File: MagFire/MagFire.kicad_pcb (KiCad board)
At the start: 2 copper layers, 1 part

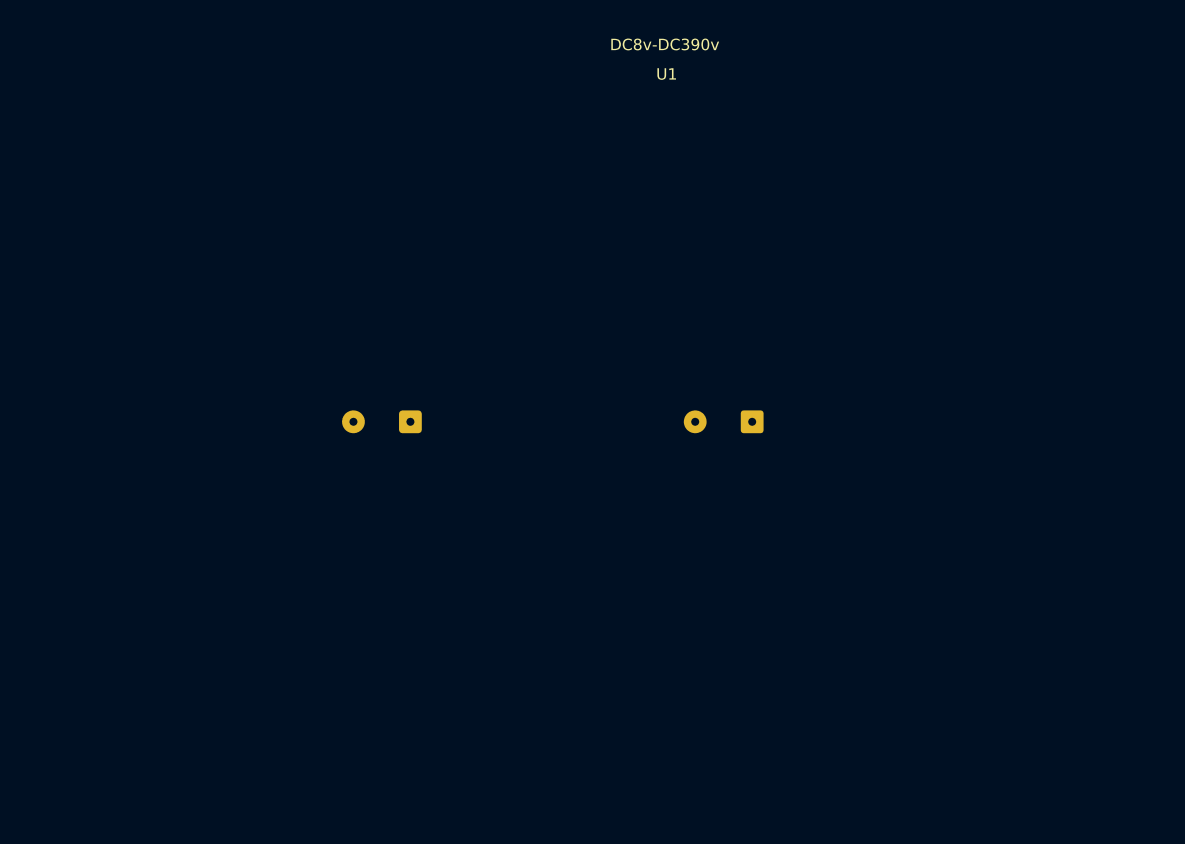
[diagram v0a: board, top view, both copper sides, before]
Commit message: update model and pcb and journal
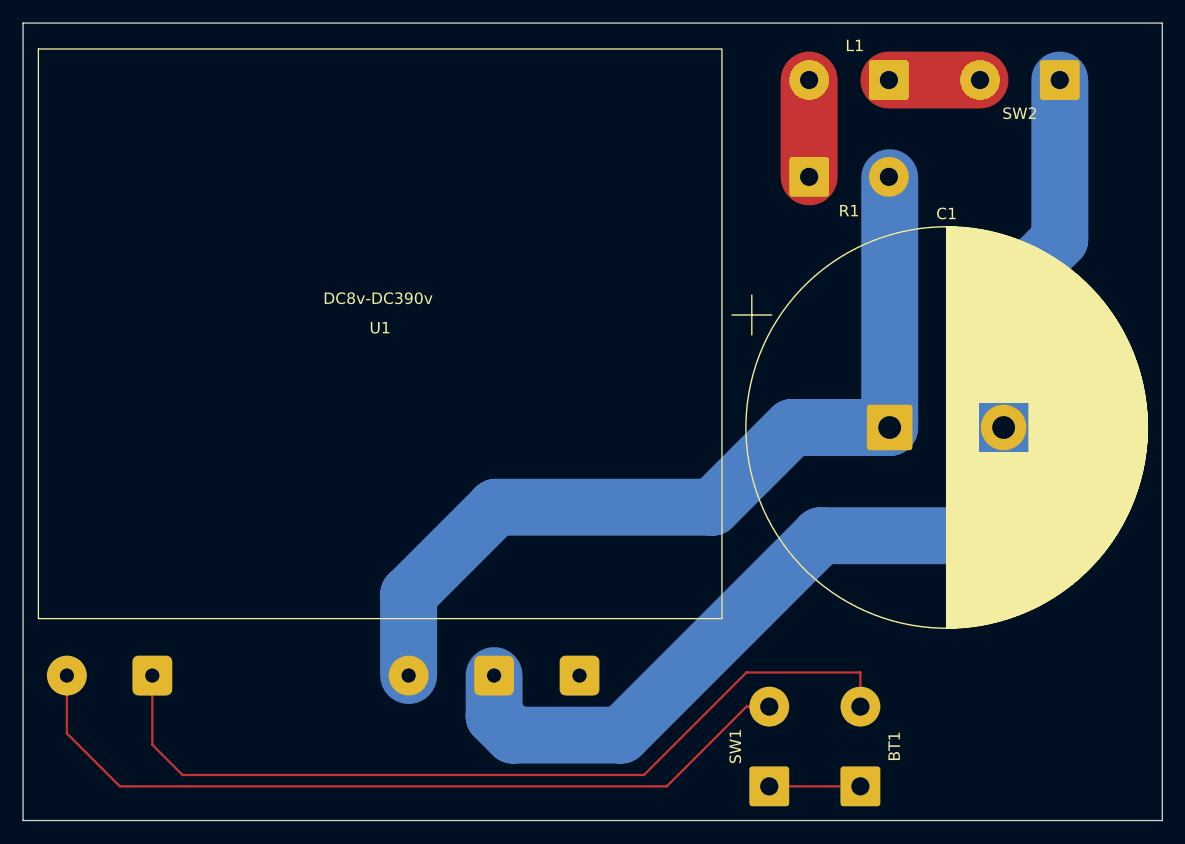
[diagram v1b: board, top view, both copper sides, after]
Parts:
- added BT1: Battery, Connector_Wire:SolderWire-0.75sqmm_1x02_P7mm_D1.25mm_OD3.5mm, F.Cu at (146.5, 142.5)
- added C1: C_US, Capacitor_THT:CP_Radial_D35.0mm_P10.00mm_SnapIn, F.Cu at (149.1, 111.0)
- added L1: L, Connector_Wire:SolderWire-0.75sqmm_1x02_P7mm_D1.25mm_OD3.5mm, F.Cu at (149.0, 80.5)
- added R1: R_US, Connector_Wire:SolderWire-0.75sqmm_1x02_P7mm_D1.25mm_OD3.5mm, F.Cu at (142.0, 89.0)
- added SW1: SW_Push, Connector_Wire:SolderWire-0.75sqmm_1x02_P7mm_D1.25mm_OD3.5mm, F.Cu at (138.5, 142.5)
- added SW2: SW_Push, Connector_Wire:SolderWire-0.75sqmm_1x02_P7mm_D1.25mm_OD3.5mm, F.Cu at (164.0, 80.5)
- U1: footprint KS_Maker:DC-DC390v_transformer_2 -> KS_Maker:DC-DC390v_transformer_3
- moved U1 33.6 mm to (104.3, 102.8)
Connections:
- U1 pad 1: unconnected-(U1-IN+-Pad1) -> Net-(U1-IN+)
- U1 pad 2: unconnected-(U1-IN--Pad2) -> Net-(BT1--)
- U1 pad 3: unconnected-(U1-OUT+-Pad3) -> Net-(U1-OUT+)
- U1 pad 4: unconnected-(U1-OUT-Pad4) -> Net-(U1-OUT)
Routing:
- net Net-(U1-OUT): track 0.00 -> 96.5 mm
- net Net-(U1-OUT+): track 0.00 -> 77.5 mm
- net Net-(BT1--): track 0.00 -> 76.5 mm
- net Net-(U1-IN+): track 0.00 -> 71.6 mm
- net Net-(L1-Pad2): track 0.00 -> 8.50 mm
- net Net-(L1-Pad1): track 0.00 -> 8.00 mm
- net Net-(BT1-+): track 0.00 -> 8.00 mm
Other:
- board outline added: 100 x 70 mm

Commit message: update everything
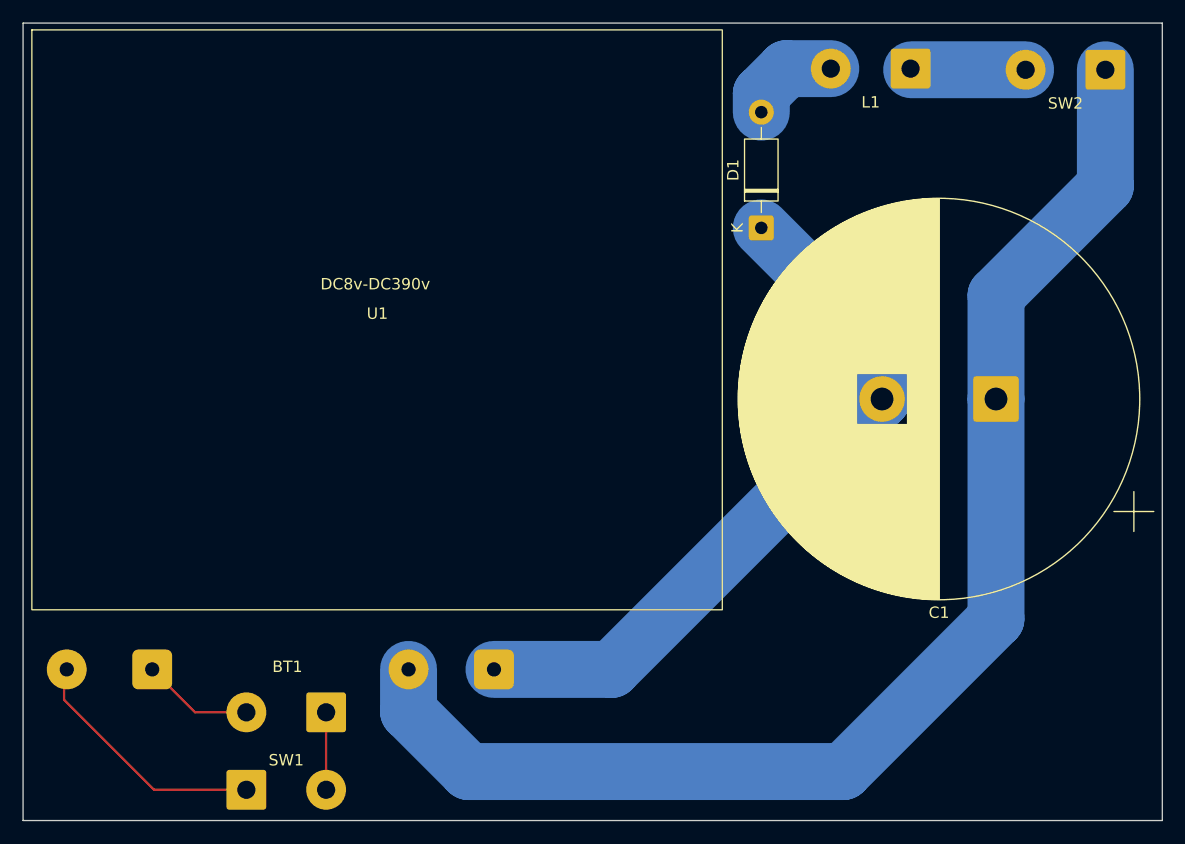
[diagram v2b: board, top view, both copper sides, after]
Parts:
- removed R1: R_US, Connector_Wire:SolderWire-0.75sqmm_1x02_P7mm_D1.25mm_OD3.5mm
- added D1: 1N4007, Diode_THT:D_DO-41_SOD81_P10.16mm_Horizontal, F.Cu at (137.8, 93.5)
- U1: footprint KS_Maker:DC-DC390v_transformer_3 -> KS_Maker:DC-DC390v_transformer_2
- moved BT1 47.3 mm to (99.6, 136.0), turned to 180 degrees
- moved SW1 45.9 mm to (92.6, 142.8), turned to 0 degrees
- moved C1 9.66 mm to (158.4, 108.5), turned to 180 degrees
- moved SW2 4.10 mm to (168.0, 79.6)
- moved L1 2.15 mm to (150.9, 79.5)
- moved U1 1.30 mm to (104.1, 101.5)
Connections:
- C1 pad 2: Net-(U1-OUT) -> Net-(D1-K)
- SW1 pad 1: Net-(BT1-+) -> Net-(U1-IN+)
- SW1 pad 2: Net-(U1-IN+) -> Net-(BT1-+)
- SW2 pad 1: Net-(U1-OUT) -> Net-(U1-OUT+)
- U1 pad 4: Net-(U1-OUT) -> Net-(D1-K)
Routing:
- net Net-(U1-OUT): track 96.5 -> 0.00 mm
- net Net-(BT1--): track 76.5 -> 9.82 mm
- net Net-(D1-K): track 0.00 -> 63.3 mm
- net Net-(U1-IN+): track 71.6 -> 22.7 mm
- net Net-(U1-OUT+): track 77.5 -> 115.2 mm
- net Net-(L1-Pad1): track 8.00 -> 10.1 mm
- net Net-(BT1-+): track 8.00 -> 6.80 mm
